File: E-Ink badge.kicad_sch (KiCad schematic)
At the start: 34 parts, among them J1 USB_C_Receptacle_USB2.0_14P, J2 E-INK-FPC, Q1 BSS138, SW1 BOOTSEL, SW2 RUN, U1 RP2040, U2 AP2112K-3.3, U3 W25Q16JVSS, Y1 Crystal

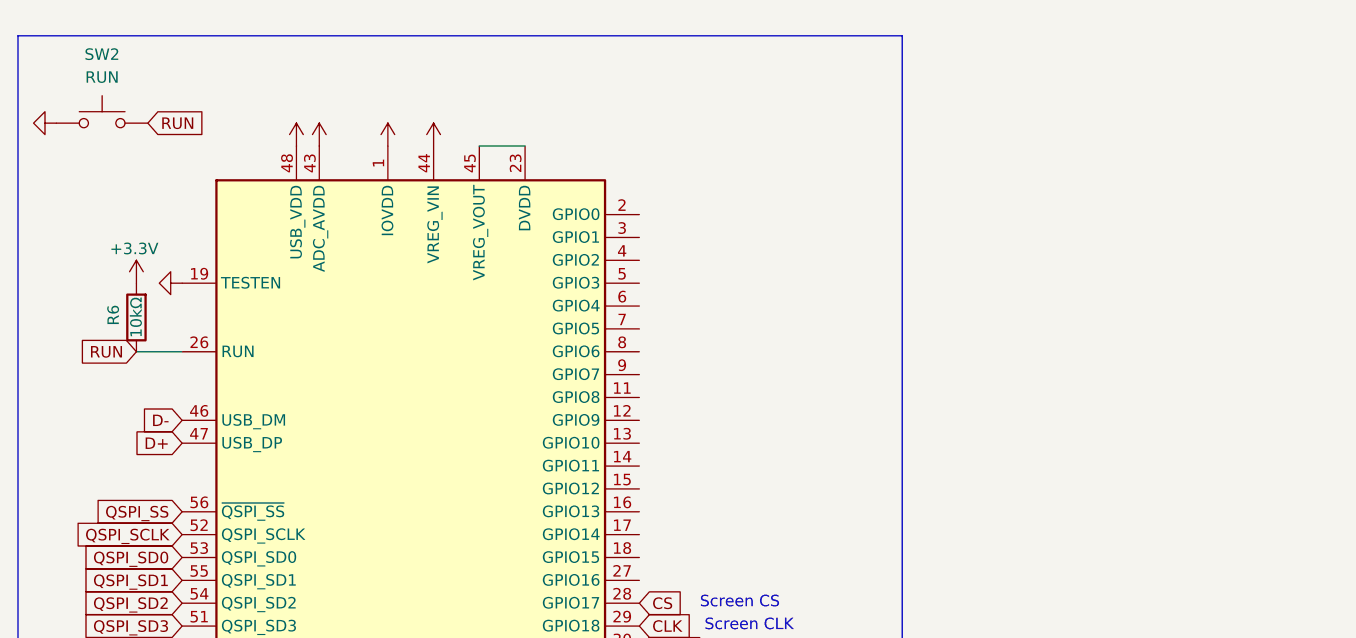
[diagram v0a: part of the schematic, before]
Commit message: Finished the main schematic besides for some pwr cutoff stuff
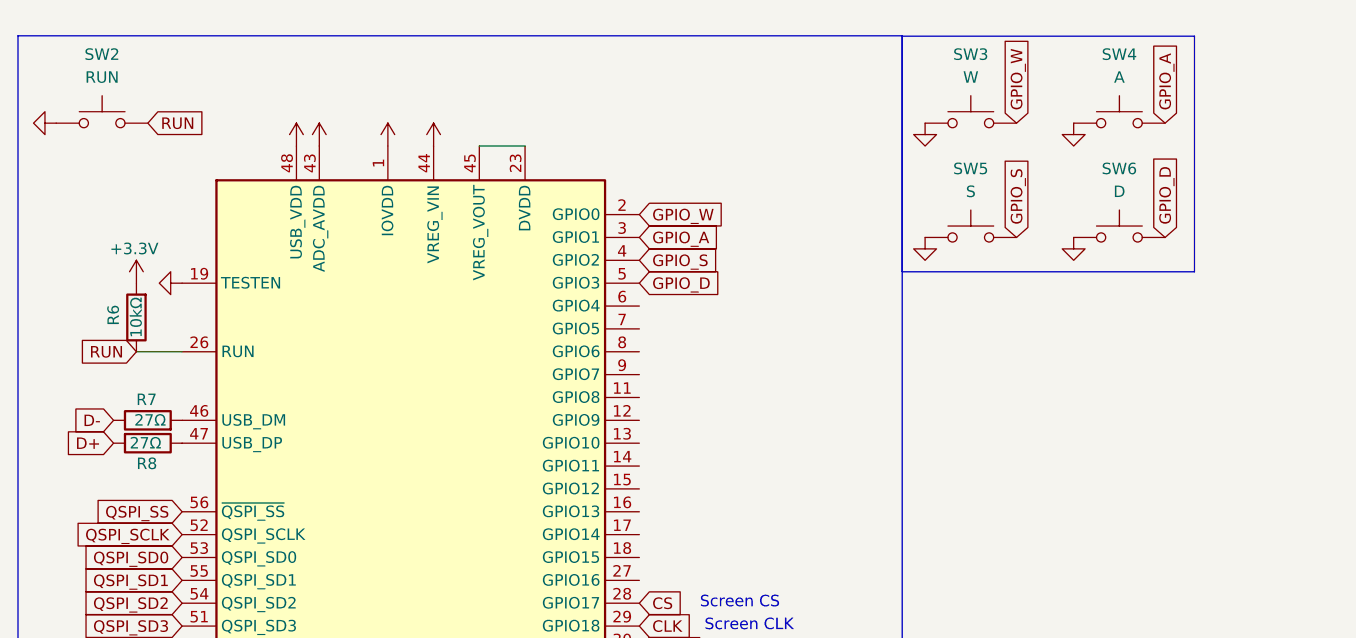
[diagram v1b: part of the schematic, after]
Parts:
- added R7, R8: 27Ω, symbol Device:R
- added SW3: W, symbol Switch:SW_Push
- added SW4: A, symbol Switch:SW_Push
- added SW5: S, symbol Switch:SW_Push
- added SW6: D, symbol Switch:SW_Push
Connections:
- net D+: now also R8.2; no longer U1.47 (USB_DP)
- net D-: now also R7.1; no longer U1.46 (USB_DM)
- net GND: now also SW3.1, SW4.1, SW5.1, SW6.1
- net GPIO_W: now reaches U1.2 (GPIO0)
- net GPIO_W: now also SW3.2
- net GPIO_A: now reaches U1.3 (GPIO1)
- net GPIO_A: now also SW4.2
- net GPIO_S: now reaches U1.4 (GPIO2)
- net GPIO_S: now also SW5.2
- net GPIO_D: now reaches U1.5 (GPIO3)
- net GPIO_D: now also SW6.2
- new net: R7.2, U1.46 (USB_DM)
- new net: R8.1, U1.47 (USB_DP)
